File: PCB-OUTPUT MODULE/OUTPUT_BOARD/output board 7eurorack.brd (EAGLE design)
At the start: 37.8 x 69.8 mm, 55 parts, among them IC1 TL072D, IC2_R TL072D, IC3_R OPA2132PA, J1 Head, J16 M05X2PTH, J2 Main, Q1_R MMBT3904, Q2_L MMBT3904

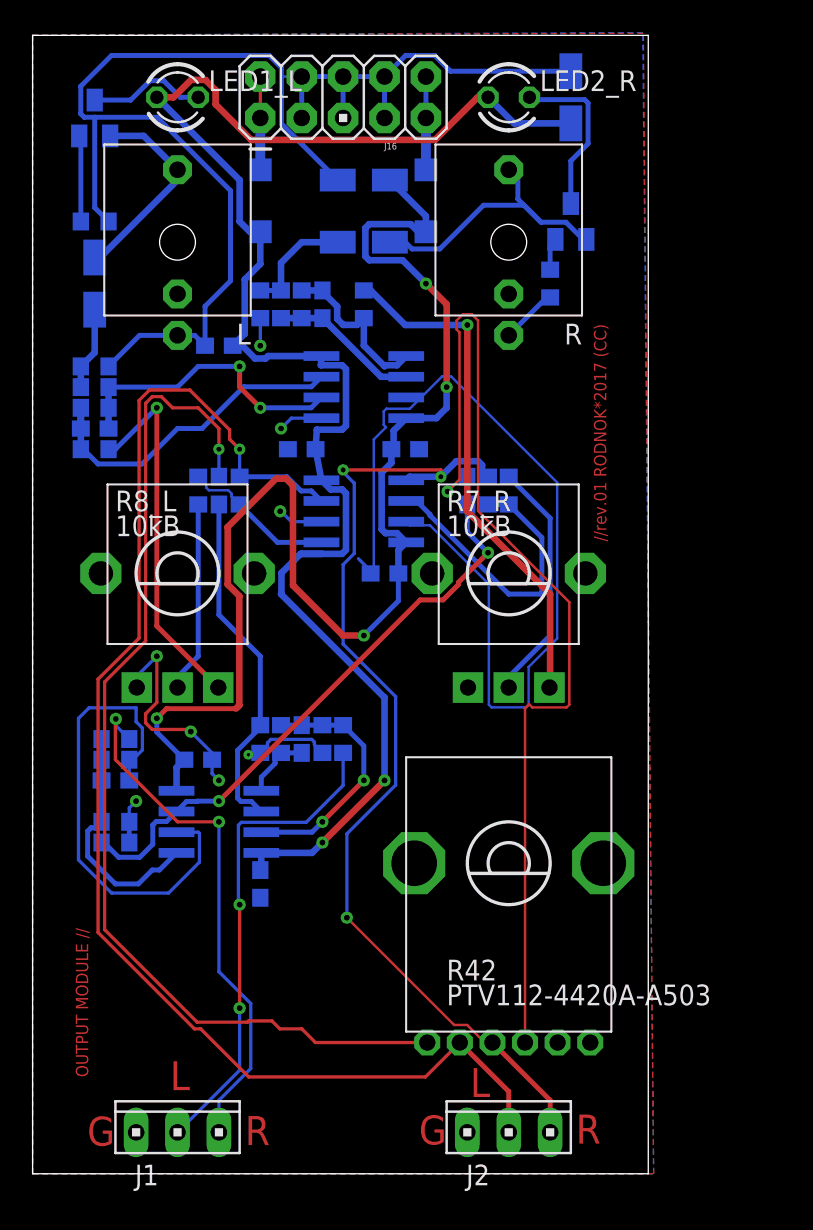
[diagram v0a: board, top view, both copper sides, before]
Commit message: Add files via upload
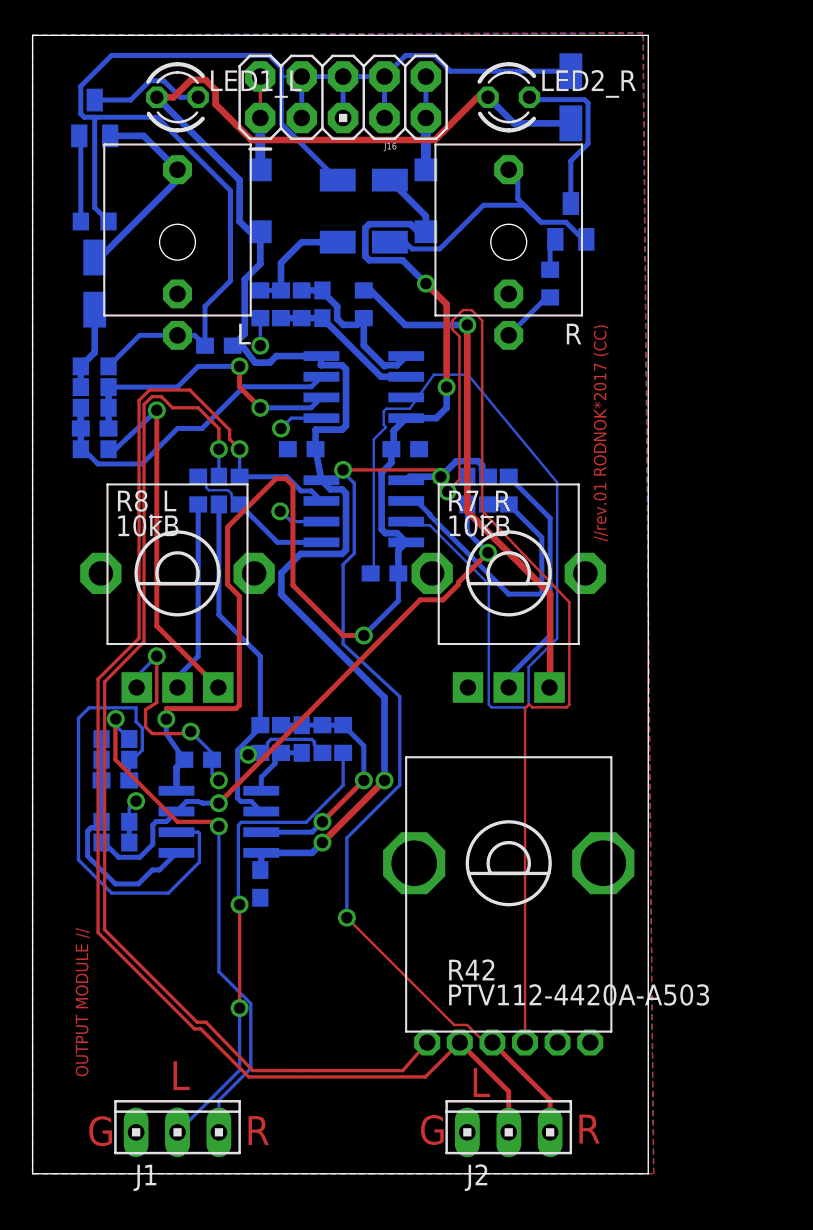
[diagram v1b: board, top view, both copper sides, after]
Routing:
- net N$16: track 64.5 -> 65.9 mm
- net VCC: track 102.2 -> 101.2 mm
- net N$26: track 63.5 -> 64.1 mm
- net VEE: track 80.3 -> 79.7 mm
